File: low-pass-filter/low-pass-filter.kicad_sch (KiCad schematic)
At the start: 38 parts, among them Q1 PNP, Q2 PNP, SW1 High Pass / Low Pass, U1 LM13700, U2 TL074, U3 TL072

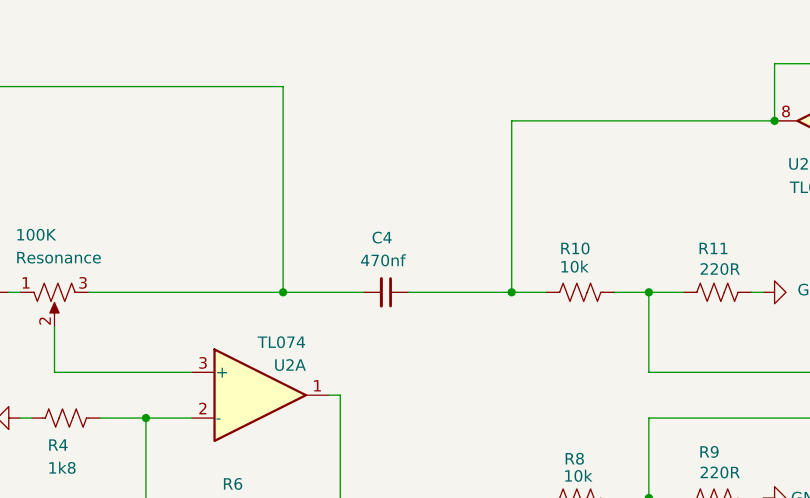
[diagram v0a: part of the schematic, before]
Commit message: Maybe fix bug in low-pass filter
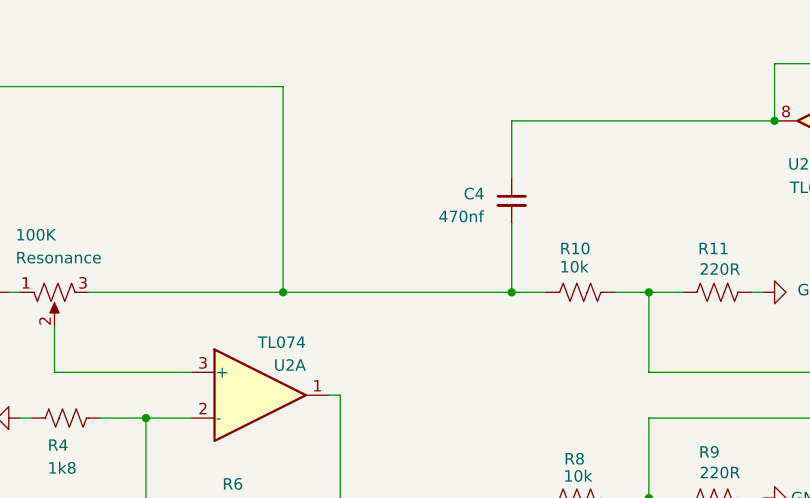
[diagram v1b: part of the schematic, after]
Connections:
- net at C4.2, R19.1, Resonance.3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: now also R10.2
- net at C4.1, U2.8, U2.9 (-): no longer R10.2
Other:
- moved on the sheet: C4
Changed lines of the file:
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@@
 	)
 	(junction
-		(at 143.51 44.45)
-		(diameter 0)
-		(color 0 0 0 0)
-	)
-	(junction
 		(at 236.22 115.57)
 		(diameter 0)
@@
 	)
 	(junction
-		(at 168.91 44.45)
-		(diameter 0)
-		(color 0 0 0 0)
-	)
-	(junction
 		(at 229.87 40.64)
 		(diameter 0)
@@
 	)
 	(junction
+		(at 143.51 44.45)
+		(diameter 0)
+		(color 0 0 0 0)
+	)
+	(junction
 		(at 97.79 44.45)
 		(diameter 0)
@@
 	)
 	(junction
+		(at 168.91 44.45)
+		(diameter 0)
+		(color 0 0 0 0)
+	)
+	(junction
 		(at 90.17 91.44)
 		(diameter 0)
@@
 	(wire
 		(pts
+			(xy 168.91 44.45) (xy 172.72 44.45)
+		)
+		(stroke
+			(width 0)
+			(type default)
+		)
+	)
+	(wire
+		(pts
 			(xy 149.86 106.68) (xy 149.86 130.81)
 		)
@@
 	(wire
 		(pts
-			(xy 168.91 44.45) (xy 157.48 44.45)
-		)
-		(stroke
-			(width 0)
-			(type default)
-		)
-	)
-	(wire
-		(pts
 			(xy 129.54 173.99) (xy 129.54 171.45)
 		)
@@
 	(wire
 		(pts
-			(xy 168.91 44.45) (xy 172.72 44.45)
+			(xy 168.91 36.83) (xy 168.91 44.45)
+		)
+		(stroke
+			(width 0)
+			(type default)
+		)
+	)
+	(wire
+		(pts
+			(xy 143.51 44.45) (xy 168.91 44.45)
 		)
 		(stroke
@@
 	(wire
 		(pts
-			(xy 213.36 19.05) (xy 198.12 19.05)
+			(xy 168.91 25.4) (xy 168.91 31.75)
 		)
 		(stroke
@@
 	(wire
 		(pts
-			(xy 236.22 83.82) (xy 236.22 95.25)
+			(xy 213.36 19.05) (xy 198.12 19.05)
 		)
 		(stroke
@@
 	(wire
 		(pts
-			(xy 219.71 115.57) (xy 224.79 115.57)
+			(xy 236.22 83.82) (xy 236.22 95.25)
 		)
 		(stroke
@@
 	(wire
 		(pts
-			(xy 36.83 120.65) (xy 34.29 120.65)
+			(xy 219.71 115.57) (xy 224.79 115.57)
 		)
 		(stroke
@@
 	(wire
 		(pts
-			(xy 243.84 143.51) (xy 243.84 140.97)
+			(xy 36.83 120.65) (xy 34.29 120.65)
 		)
 		(stroke
@@
 	(wire
 		(pts
-			(xy 184.15 44.45) (xy 187.96 44.45)
+			(xy 243.84 143.51) (xy 243.84 140.97)
 		)
 		(stroke
@@
 	(wire
 		(pts
-			(xy 34.29 120.65) (xy 31.75 120.65)
+			(xy 184.15 44.45) (xy 187.96 44.45)
 		)
 		(stroke
@@
 	(wire
 		(pts
-			(xy 128.27 97.79) (xy 133.35 97.79)
+			(xy 34.29 120.65) (xy 31.75 120.65)
 		)
 		(stroke
@@
 	(wire
 		(pts
-			(xy 143.51 44.45) (xy 152.4 44.45)
+			(xy 128.27 97.79) (xy 133.35 97.79)
 		)
 		(stroke
@@
 	(wire
 		(pts
-			(xy 168.91 25.4) (xy 168.91 44.45)
-		)
-		(stroke
-			(width 0)
-			(type default)
-		)
-	)
-	(wire
-		(pts
 			(xy 97.79 88.9) (xy 97.79 91.44)
 		)
@@
 		)
 		(instances
-			(project ""
+			(project "low-pass-filter"
 				(path "/e72ee090-6f9b-4823-9ab6-f31beee51bd1"
 					(reference "U3")
@@
 		)
 		(instances
-			(project ""
+			(project "low-pass-filter"
 				(path "/e72ee090-6f9b-4823-9ab6-f31beee51bd1"
 					(reference "U3")
@@
 	(symbol
 		(lib_id "Device:C_Small")
-		(at 154.94 44.45 270)
+		(at 168.91 34.29 0)
 		(unit 1)
 		(exclude_from_sim no)
@@
 		(dnp no)
 		(property "Reference" "C4"
-			(at 153.3525 38.4175 90)
+			(at 163.576 33.528 0)
 			(effects
 				(font
@@
 		)
 		(property "Value" "470nf"
-			(at 152.0825 40.9575 90)
+			(at 160.782 36.068 0)
 			(effects
 				(font
@@
 		)
 		(property "Footprint" ""
-			(at 154.94 44.45 0)
+			(at 168.91 34.29 0)
 			(effects
 				(font
@@
 		)
 		(property "Datasheet" "~"
-			(at 154.94 44.45 0)
+			(at 168.91 34.29 0)
 			(effects
 				(font
@@
 		)
 		(property "Description" ""
-			(at 154.94 44.45 0)
+			(at 168.91 34.29 0)
 			(effects
 				(font
@@
 		)
 		(instances
-			(project ""
+			(project "low-pass-filter"
 				(path "/e72ee090-6f9b-4823-9ab6-f31beee51bd1"
 					(reference "SW1")
@@
 		)
 		(instances
-			(project ""
+			(project "low-pass-filter"
 				(path "/e72ee090-6f9b-4823-9ab6-f31beee51bd1"
 					(reference "#PWR023")
@@
 		)
 		(instances
-			(project ""
+			(project "low-pass-filter"
 				(path "/e72ee090-6f9b-4823-9ab6-f31beee51bd1"
 					(reference "U3")

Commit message: Revert "Maybe fix bug in low-pass filter"
It was right the first time.

This reverts commit b62497d0d33f661917a797e78c2c214d61ac51a2.
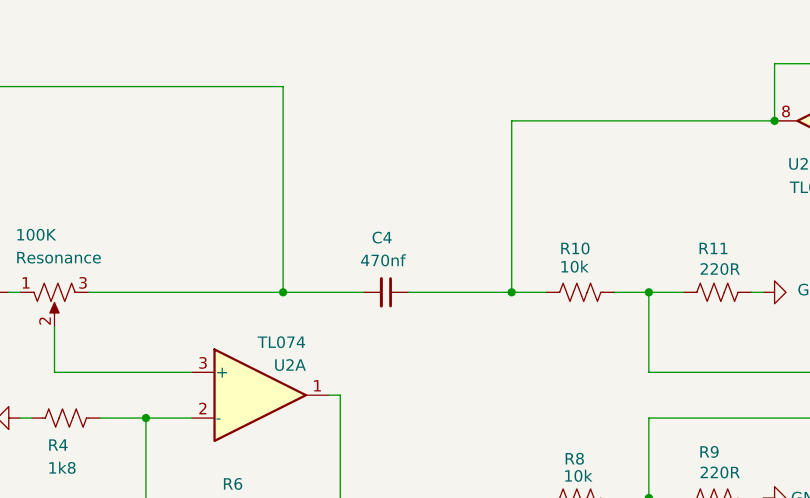
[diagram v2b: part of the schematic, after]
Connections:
- net at C4.2, R19.1, Resonance.3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: no longer R10.2
- net at C4.1, U2.8, U2.9 (-): now also R10.2
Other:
- moved on the sheet: C4
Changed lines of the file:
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@@
 	)
 	(junction
+		(at 143.51 44.45)
+		(diameter 0)
+		(color 0 0 0 0)
+	)
+	(junction
 		(at 236.22 115.57)
 		(diameter 0)
@@
 	)
 	(junction
+		(at 168.91 44.45)
+		(diameter 0)
+		(color 0 0 0 0)
+	)
+	(junction
 		(at 229.87 40.64)
 		(diameter 0)
@@
 	)
 	(junction
-		(at 143.51 44.45)
-		(diameter 0)
-		(color 0 0 0 0)
-	)
-	(junction
 		(at 97.79 44.45)
 		(diameter 0)
@@
 	)
 	(junction
-		(at 168.91 44.45)
-		(diameter 0)
-		(color 0 0 0 0)
-	)
-	(junction
 		(at 90.17 91.44)
 		(diameter 0)
@@
 	(wire
 		(pts
-			(xy 168.91 44.45) (xy 172.72 44.45)
-		)
-		(stroke
-			(width 0)
-			(type default)
-		)
-	)
-	(wire
-		(pts
 			(xy 149.86 106.68) (xy 149.86 130.81)
 		)
@@
 	(wire
 		(pts
+			(xy 168.91 44.45) (xy 157.48 44.45)
+		)
+		(stroke
+			(width 0)
+			(type default)
+		)
+	)
+	(wire
+		(pts
 			(xy 129.54 173.99) (xy 129.54 171.45)
 		)
@@
 	(wire
 		(pts
-			(xy 168.91 36.83) (xy 168.91 44.45)
-		)
-		(stroke
-			(width 0)
-			(type default)
-		)
-	)
-	(wire
-		(pts
-			(xy 143.51 44.45) (xy 168.91 44.45)
+			(xy 168.91 44.45) (xy 172.72 44.45)
 		)
 		(stroke
@@
 	(wire
 		(pts
-			(xy 168.91 25.4) (xy 168.91 31.75)
-		)
-		(stroke
-			(width 0)
-			(type default)
-		)
-	)
-	(wire
-		(pts
 			(xy 213.36 19.05) (xy 198.12 19.05)
 		)
@@
 	(wire
 		(pts
+			(xy 143.51 44.45) (xy 152.4 44.45)
+		)
+		(stroke
+			(width 0)
+			(type default)
+		)
+	)
+	(wire
+		(pts
 			(xy 74.93 60.96) (xy 74.93 84.7725)
 		)
@@
 	(wire
 		(pts
+			(xy 168.91 25.4) (xy 168.91 44.45)
+		)
+		(stroke
+			(width 0)
+			(type default)
+		)
+	)
+	(wire
+		(pts
 			(xy 97.79 88.9) (xy 97.79 91.44)
 		)
@@
 		)
 		(instances
-			(project "low-pass-filter"
+			(project ""
 				(path "/e72ee090-6f9b-4823-9ab6-f31beee51bd1"
 					(reference "U3")
@@
 		)
 		(instances
-			(project "low-pass-filter"
+			(project ""
 				(path "/e72ee090-6f9b-4823-9ab6-f31beee51bd1"
 					(reference "U3")
@@
 	(symbol
 		(lib_id "Device:C_Small")
-		(at 168.91 34.29 0)
+		(at 154.94 44.45 270)
 		(unit 1)
 		(exclude_from_sim no)
@@
 		(dnp no)
 		(property "Reference" "C4"
-			(at 163.576 33.528 0)
+			(at 153.3525 38.4175 90)
 			(effects
 				(font
@@
 		)
 		(property "Value" "470nf"
-			(at 160.782 36.068 0)
+			(at 152.0825 40.9575 90)
 			(effects
 				(font
@@
 		)
 		(property "Footprint" ""
-			(at 168.91 34.29 0)
+			(at 154.94 44.45 0)
 			(effects
 				(font
@@
 		)
 		(property "Datasheet" "~"
-			(at 168.91 34.29 0)
+			(at 154.94 44.45 0)
 			(effects
 				(font
@@
 		)
 		(property "Description" ""
-			(at 168.91 34.29 0)
+			(at 154.94 44.45 0)
 			(effects
 				(font
@@
 		)
 		(instances
-			(project "low-pass-filter"
+			(project ""
 				(path "/e72ee090-6f9b-4823-9ab6-f31beee51bd1"
 					(reference "SW1")
@@
 		)
 		(instances
-			(project "low-pass-filter"
+			(project ""
 				(path "/e72ee090-6f9b-4823-9ab6-f31beee51bd1"
 					(reference "#PWR023")
@@
 		)
 		(instances
-			(project "low-pass-filter"
+			(project ""
 				(path "/e72ee090-6f9b-4823-9ab6-f31beee51bd1"
 					(reference "U3")
